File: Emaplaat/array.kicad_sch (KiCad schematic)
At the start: 29 parts, among them U1 1EDN7550BXTSA1

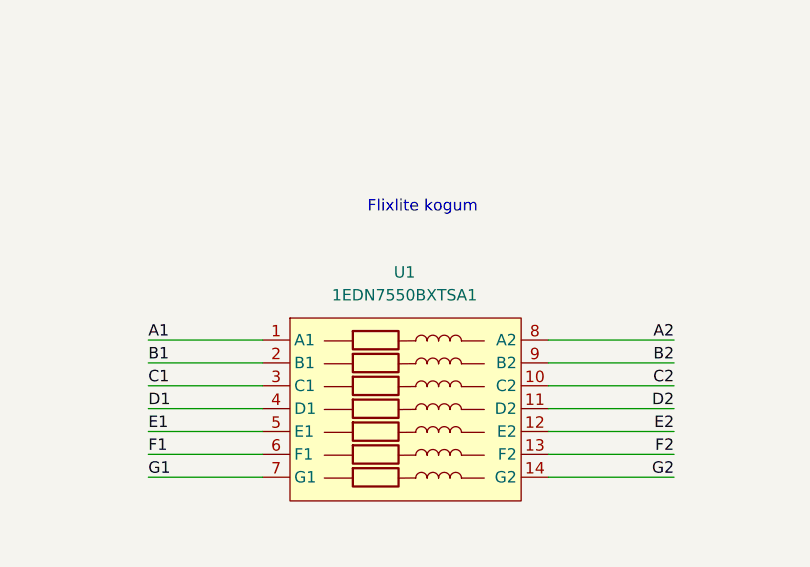
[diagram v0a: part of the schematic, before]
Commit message: v3.3 Abeltoni tagasiside veelkord
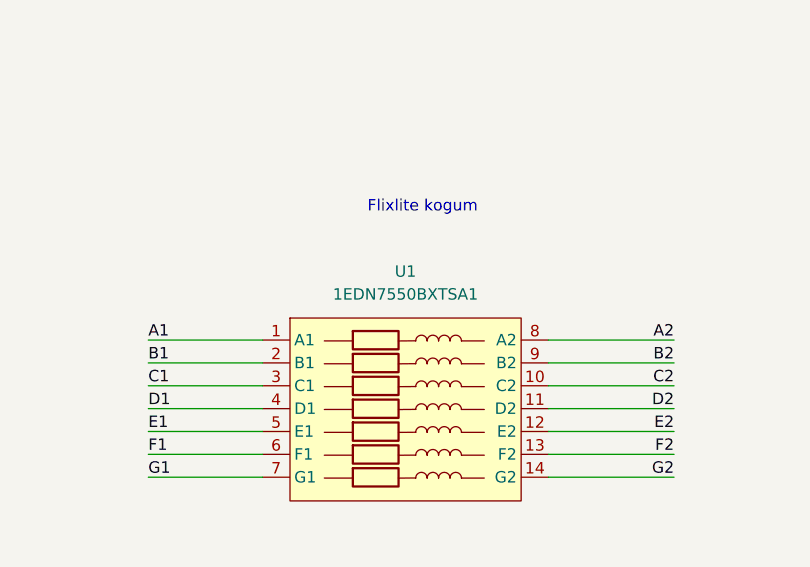
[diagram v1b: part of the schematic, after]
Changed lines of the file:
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@@
 		(fields_autoplaced yes)
 		(property "Reference" "U1"
-			(at 165.6293 78.8353 0)
+			(at 165.735 78.74 0)
 			(effects
 				(font
@@
 		)
 		(property "Value" "1EDN7550BXTSA1"
-			(at 165.6293 81.3753 0)
+			(at 165.735 81.28 0)
 			(effects
 				(font
